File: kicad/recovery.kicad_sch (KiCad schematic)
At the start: 50 parts, among them J1 Bus_PCI_Express_x1, J2 wago 2060-452/998-404, J3 wago 2060-452/998-404, J4 Conn_01x04, J5 Conn_01x02_Pin, J6 USB_C_Receptacle_USB2.0_16P, Q1 SI7232DN-T1-GE3, U2 RP2040, U4 W25Q128JVP, U9 MCP25625T-E/ML, X1 RP2040 Crystal, Y2 X322516MLB4SI

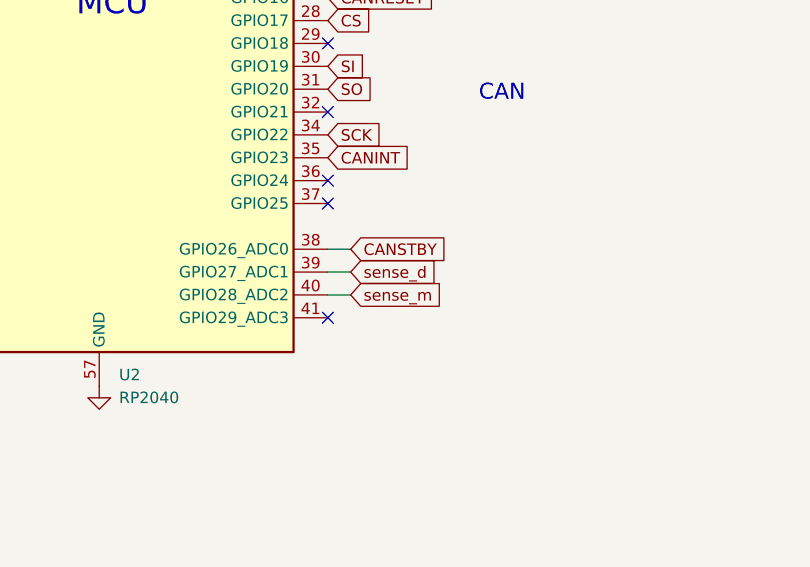
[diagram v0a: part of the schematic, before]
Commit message: finish routing
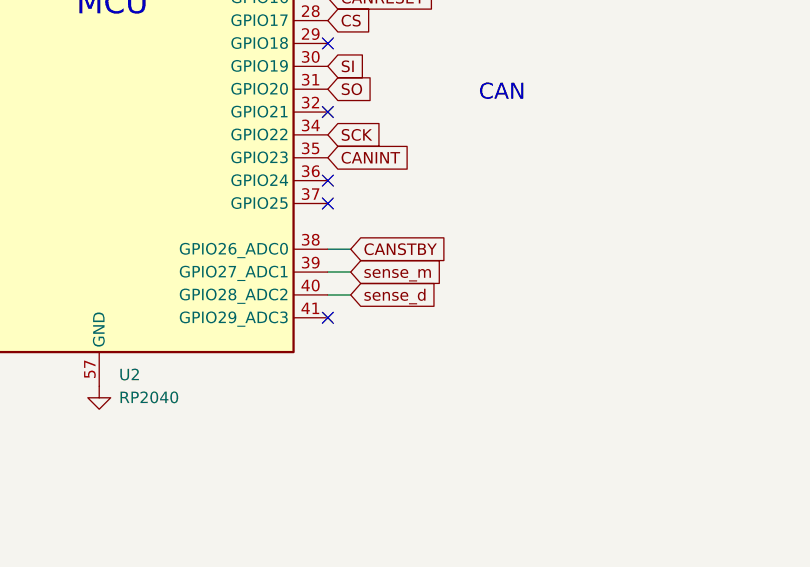
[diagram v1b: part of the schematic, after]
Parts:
- J1: footprint Connector_PCBEdge:BUS_PCIexpress_x1 -> 4in-kicad-library:PCIeX1
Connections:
- net sense_d: now also U2.40 (GPIO28_ADC2); no longer U2.39 (GPIO27_ADC1)
- net sense_m: now also U2.39 (GPIO27_ADC1); no longer U2.40 (GPIO28_ADC2)
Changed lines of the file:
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@@
 	(global_label "sense_m"
 		(shape input)
-		(at 327.66 217.17 0)
+		(at 327.66 214.63 0)
 		(fields_autoplaced yes)
 		(effects
@@
 		)
 		(property "Intersheetrefs" "${INTERSHEET_REFS}"
-			(at 338.6885 217.17 0)
+			(at 338.6885 214.63 0)
 			(effects
 				(font
@@
 	(global_label "sense_d"
 		(shape input)
-		(at 327.66 214.63 0)
+		(at 327.66 217.17 0)
 		(fields_autoplaced yes)
 		(effects
@@
 		)
 		(property "Intersheetrefs" "${INTERSHEET_REFS}"
-			(at 338.1442 214.63 0)
+			(at 338.1442 217.17 0)
 			(effects
 				(font
@@
 			)
 		)
-		(property "Footprint" "Connector_PCBEdge:BUS_PCIexpress_x1"
+		(property "Footprint" "4in-kicad-library:PCIeX1"
 			(at 74.93 261.62 0)
 			(effects
